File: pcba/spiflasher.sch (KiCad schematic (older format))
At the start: 41 parts, among them J1 USB_B_Micro, J2 Conn_02x04_Counter_Clockwise, J3 Conn_01x10, J4 Conn_01x10, U1 FT232H, U2 93LC56BT-I/OT, U3 TXB0104PW, Y1 12 MHz

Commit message: Changed crystal Digikey P/N to a non-marketplace one
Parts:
- Y1: Digikey 2388-SXT32420AA07-12.000M-ND -> XC2911CT-ND
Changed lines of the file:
@@
 F 3 "~" H 4250 4750 50  0001 C CNN
 F 4 "C9002" H 4250 4750 50  0001 C CNN "LCSC"
-F 5 " 2388-SXT32420AA07-12.000M-ND " H 4250 4750 50  0001 C CNN "Digikey"
+F 5 " XC2911CT-ND " H 4250 4750 50  0001 C CNN "Digikey"
 	1    4250 4750
 	0    1    1    0

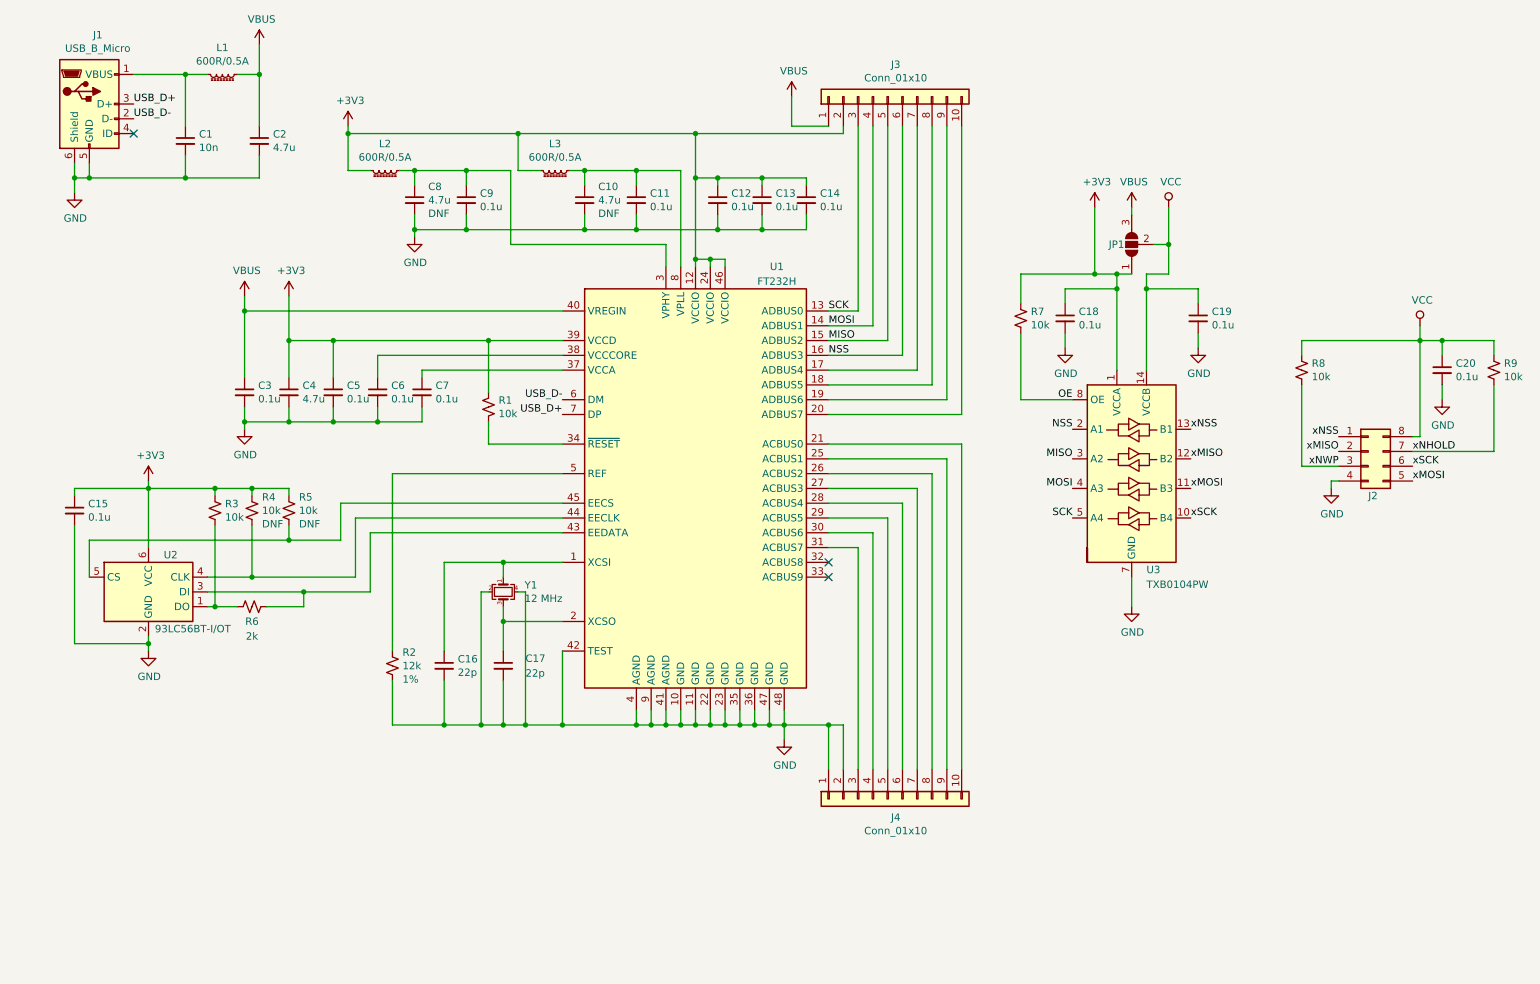
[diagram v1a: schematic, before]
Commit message: Removed unnecessary components.
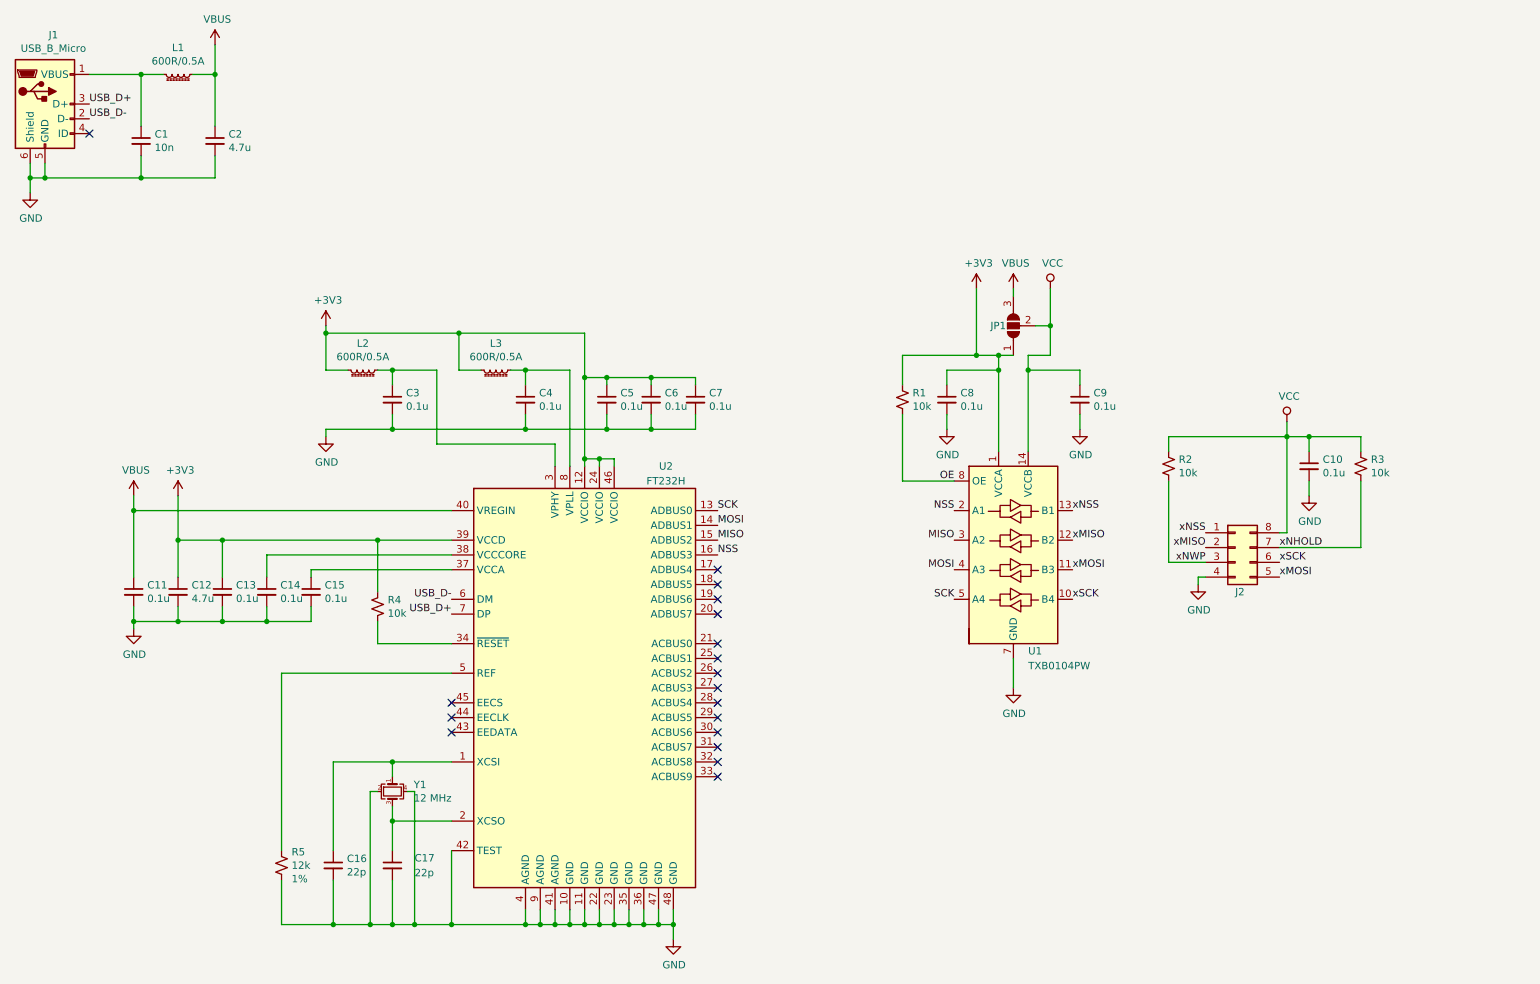
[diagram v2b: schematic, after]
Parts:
- removed C10, C8: 4.7u, Capacitor_SMD:C_0603_1608Metric, symbol Device:C_Small
- removed C15: 0.1u, Capacitor_SMD:C_0603_1608Metric, symbol Device:C_Small
- removed J3, J4: Conn_01x10, Connector_PinHeader_2.54mm:PinHeader_1x10_P2.54mm_Vertical, symbol Connector_Generic:Conn_01x10
- removed R3, R4, R5: 10k, Resistor_SMD:R_0603_1608Metric, symbol Device:R_Small_US
- removed R6: 2k, Resistor_SMD:R_0603_1608Metric, symbol Device:R_Small_US
- removed U2: 93LC56BT-I/OT, Package_TO_SOT_SMD:SOT-23-6, symbol Memory_EEPROM:93LCxxBxxOT
- Y1: footprint Crystal:Crystal_SMD_3225-4Pin_3.2x2.5mm_HandSoldering -> Crystal:Crystal_SMD_3225-4Pin_3.2x2.5mm
- renumbered C20 to C10, C3 to C11, C4 to C12, C5 to C13, C6 to C14, C7 to C15, C9 to C3, C11 to C4, C12 to C5, C13 to C6, C14 to C7, C18 to C8, C19 to C9, R7 to R1, R8 to R2, R9 to R3, R1 to R4, R2 to R5, U3 to U1, U1 to U2
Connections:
- no-connect marks 3 -> 18
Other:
- moved on the sheet: C1, C10, C11, C12, C13, C14, C15, C16, C17, C2, C3, C4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
